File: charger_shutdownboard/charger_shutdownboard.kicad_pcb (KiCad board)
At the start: 2 copper layers, 53.5 x 58 mm, 18 parts, among them J1 Conn_01x08_Pin, J2 Conn_01x02_Pin, J3 Conn_01x02_Pin, J4 Conn_01x02_Pin, J5 Conn_01x02_Pin, J6 Conn_01x02_Pin, J7 Conn_01x02_Pin

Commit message: value for voltage divider resistors for bspd_fault changed
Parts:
- R1: value 70k -> 68k
- R2: value 50k -> 47k
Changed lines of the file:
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@@
 		)
 		(fp_text user "${REFERENCE}"
-			(at 3.54 6.25 360)
+			(at 3.54 6.25 0)
 			(layer "F.Fab")
 			(effects
@@
 		(tags "connector Molex Nano-Fit side entry")
 		(property "Reference" "J4"
-			(at 0 -2.92 360)
+			(at 0 -2.92 0)
 			(layer "F.SilkS")
 			(effects
@@
 		)
 		(property "Value" "Conn_01x02_Pin"
-			(at 0 5.42 360)
+			(at 0 5.42 0)
 			(layer "F.Fab")
 			(effects
@@
 			)
 		)
-		(property "Value" "70k"
+		(property "Value" "68k"
 			(at 0 1.65 0)
 			(layer "F.Fab")
@@
 		(tags "connector Molex Nano-Fit side entry")
 		(property "Reference" "J3"
-			(at 0 -2.92 360)
+			(at 0 -2.92 0)
 			(layer "F.SilkS")
 			(effects
@@
 		)
 		(property "Value" "Conn_01x02_Pin"
-			(at 0 5.42 360)
+			(at 0 5.42 0)
 			(layer "F.Fab")
 			(effects
@@
 		(tags "resistor handsolder")
 		(property "Reference" "R4"
-			(at 0 -2 360)
+			(at 0 -2 0)
 			(layer "F.SilkS")
 			(effects
@@
 		)
 		(property "Value" "38k"
-			(at 0 1.65 360)
+			(at 0 1.65 0)
 			(layer "F.Fab")
 			(effects
@@
 		)
 		(fp_text user "${REFERENCE}"
-			(at 0 0 360)
+			(at 0 0 0)
 			(layer "F.Fab")
 			(effects
@@
 		)
 		(fp_text user "${REFERENCE}"
-			(at 1.1 1.25 360)
+			(at 1.1 1.25 0)
 			(layer "F.Fab")
 			(effects
@@
 		(tags "resistor handsolder")
 		(property "Reference" "R2"
-			(at 0 -2 360)
+			(at 0 -2 0)
 			(layer "F.SilkS")
 			(effects
@@
 			)
 		)
-		(property "Value" "50k"
-			(at 0 1.65 360)
+		(property "Value" "47k"
+			(at 0 1.65 0)
 			(layer "F.Fab")
 			(effects
@@
 		)
 		(fp_text user "${REFERENCE}"
-			(at 0 0 360)
+			(at 0 0 0)
 			(layer "F.Fab")
 			(effects
@@
 		(tags "connector Molex Nano-Fit side entry")
 		(property "Reference" "J6"
-			(at 0 -2.92 360)
+			(at 0 -2.92 0)
 			(layer "F.SilkS")
 			(effects
@@
 		)
 		(property "Value" "Conn_01x02_Pin"
-			(at 0 5.42 360)
+			(at 0 5.42 0)
 			(layer "F.Fab")
 			(effects

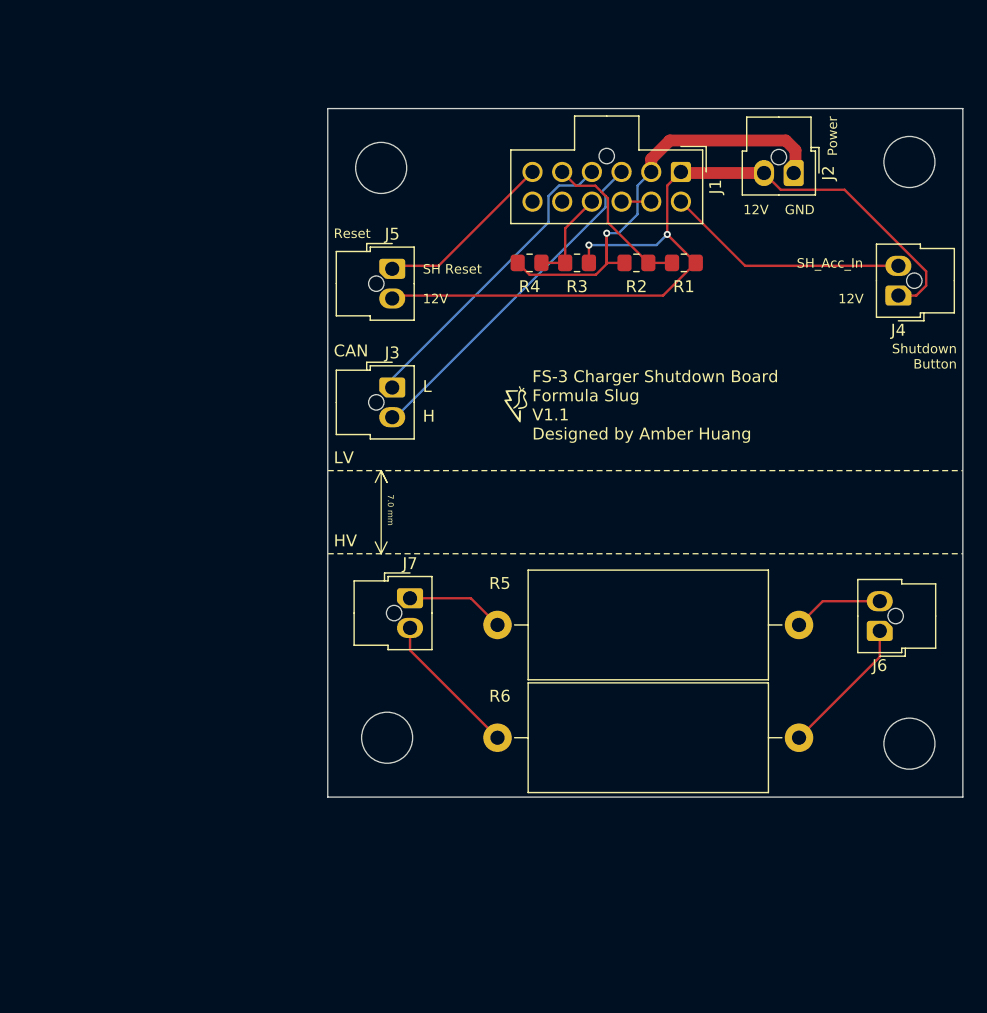
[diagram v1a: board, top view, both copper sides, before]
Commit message: Revised PCB for J1772 negotiation
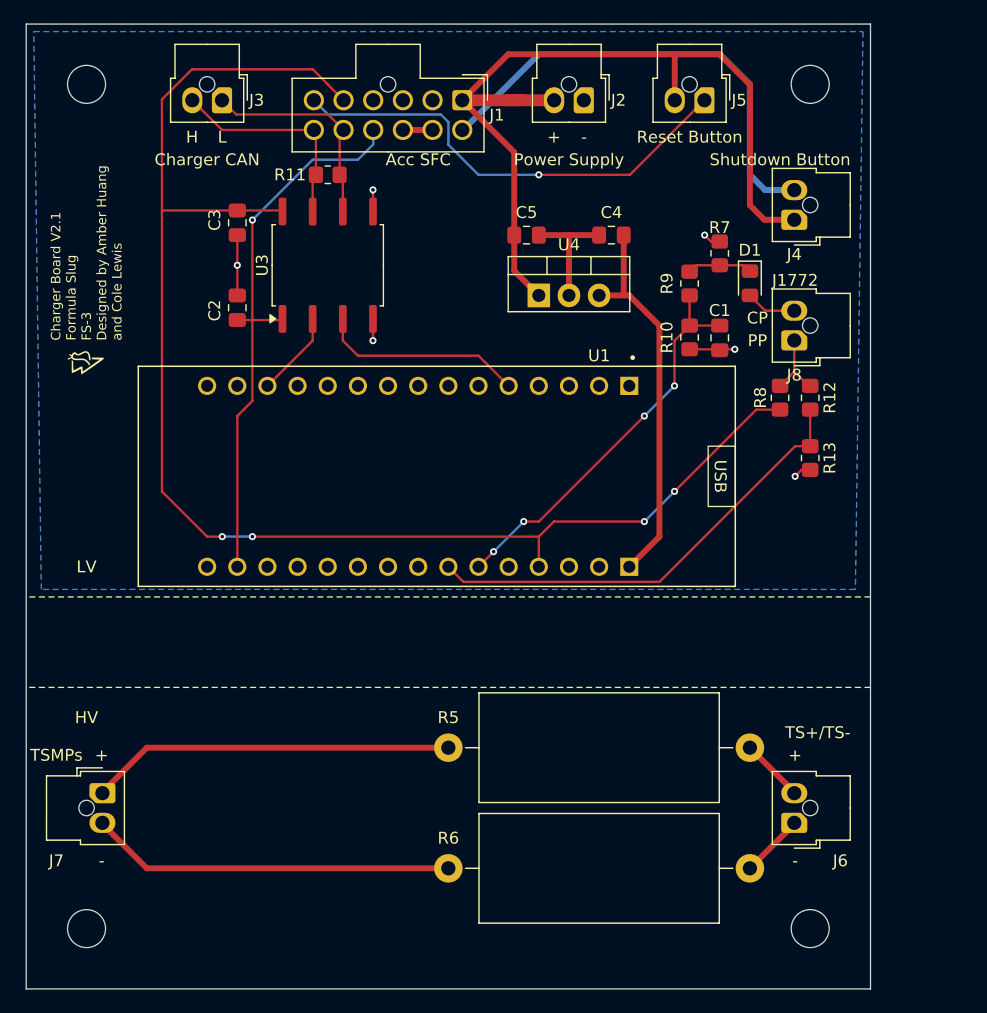
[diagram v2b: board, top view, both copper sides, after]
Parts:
- removed R1: 68k, Resistor_SMD:R_0805_2012Metric_Pad1.20x1.40mm_HandSolder
- removed R2: 47k, Resistor_SMD:R_0805_2012Metric_Pad1.20x1.40mm_HandSolder
- removed R3: 100k, Resistor_SMD:R_0805_2012Metric_Pad1.20x1.40mm_HandSolder
- removed R4: 38k, Resistor_SMD:R_0805_2012Metric_Pad1.20x1.40mm_HandSolder
- removed the REF** at (176.0, 116.5)
- removed the REF** at (132.0, 116.0)
- removed the REF** at (131.5, 68.0)
- removed the REF** at (176.0, 67.5)
- added C1: 100nF, Capacitor_SMD:C_0805_2012Metric_Pad1.18x1.45mm_HandSolder, F.Cu at (160.0, 82.3)
- added C2: 100nF, Capacitor_SMD:C_0805_2012Metric_Pad1.18x1.45mm_HandSolder, F.Cu at (119.4, 79.8)
- added C3: 100nF, Capacitor_SMD:C_0805_2012Metric_Pad1.18x1.45mm_HandSolder, F.Cu at (119.4, 72.6)
- added C4: 100nF, Capacitor_SMD:C_0805_2012Metric_Pad1.18x1.45mm_HandSolder, F.Cu at (150.9, 73.7)
- added C5: 100nF, Capacitor_SMD:C_0805_2012Metric_Pad1.18x1.45mm_HandSolder, F.Cu at (143.7, 73.7)
- added D1: D, Diode_SMD:D_0805_2012Metric_Pad1.15x1.40mm_HandSolder, F.Cu at (162.6, 77.7)
- added J8: J1772, Connector_Molex:Molex_Nano-Fit_105309-xx02_1x02_P2.50mm_Vertical, F.Cu at (166.3, 82.5)
- added R10: 499k, Resistor_SMD:R_0805_2012Metric_Pad1.20x1.40mm_HandSolder, F.Cu at (157.5, 82.3)
- added R11: 120, Resistor_SMD:R_0805_2012Metric_Pad1.20x1.40mm_HandSolder, F.Cu at (127.0, 68.6)
- added R12: 200k, Resistor_SMD:R_0805_2012Metric_Pad1.20x1.40mm_HandSolder, F.Cu at (167.6, 87.4)
- added R13: 330k, Resistor_SMD:R_0805_2012Metric_Pad1.20x1.40mm_HandSolder, F.Cu at (167.6, 92.4)
- added R7: 866, Resistor_SMD:R_0805_2012Metric_Pad1.20x1.40mm_HandSolder, F.Cu at (160.0, 75.2)
- added R8: 330, Resistor_SMD:R_0805_2012Metric_Pad1.20x1.40mm_HandSolder, F.Cu at (165.1, 87.4)
- added R9: 330k, Resistor_SMD:R_0805_2012Metric_Pad1.20x1.40mm_HandSolder, F.Cu at (157.5, 77.7)
- added REF**: MountingHole_3.2mm_M3, MountingHole:MountingHole_3.2mm_M3, F.Cu at (106.7, 132.1)
- added REF**: MountingHole_3.2mm_M3, MountingHole:MountingHole_3.2mm_M3, F.Cu at (167.6, 61.0)
- added REF**: MountingHole_3.2mm_M3, MountingHole:MountingHole_3.2mm_M3, F.Cu at (167.6, 132.1)
- added REF**: MountingHole_3.2mm_M3, MountingHole:MountingHole_3.2mm_M3, F.Cu at (106.7, 61.0)
- added U1: NUCLEO-L432KC, FS_3_Global_Footprint_Library:NUCLEO-L432KC, F.Cu at (136.2, 94.0)
- added U3: ISO1050DUB, Package_SO:SOP-8_6.62x9.15mm_P2.54mm, F.Cu at (127.0, 76.2)
- added U4: LM7809_TO220, Package_TO_SOT_THT:TO-220-3_Vertical, F.Cu at (144.8, 78.7)
- J1: value Conn_01x08_Pin -> Acc SFC
- J2: value Conn_01x02_Pin -> Power Supply
- J3: value Conn_01x02_Pin -> Charger CAN
- J4: value Conn_01x02_Pin -> Shutdown Button
- J5: value Conn_01x02_Pin -> Reset Button
- J6: value Conn_01x02_Pin -> TS+/TS-
- J7: value Conn_01x02_Pin -> TSMPs
- moved G*** 39.9 mm to (106.7, 81.2), turned to 90 degrees
- moved J7 30.7 mm to (108.0, 120.7)
- moved J5 29.9 mm to (158.7, 62.3), turned to -90 degrees
- moved J3 28.1 mm to (118.1, 62.3), turned to -90 degrees
- moved J1 19.4 mm to (138.3, 62.3)
- moved J2 18.7 mm to (148.6, 62.3)
- moved J6 17.7 mm to (166.3, 123.2)
- moved R6 11.8 mm to (137.2, 127.0)
- moved R5 11.1 mm to (137.2, 116.8)
- moved J4 10.8 mm to (166.3, 72.4)
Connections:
- J1 pad 10: /Charge_State -> +3V3
- J1 pad 11: unconnected-(J1-Pin_11-Pad11) -> /CAN_L
- J1 pad 12: unconnected-(J1-Pin_12-Pad12) -> /CAN_H
- J1 pad 3: /CAN_H -> unconnected-(J1-Pin_3-Pad3)
- J1 pad 4: /CAN_L -> unconnected-(J1-Pin_4-Pad4)
- J1 pad 5: /BSPD_fault -> +5V
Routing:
- net +5V: track 0.00 -> 121.1 mm, vias 0 -> 4
- net +3V3: track 0.00 -> 47.5 mm, vias 0 -> 1
- net /Proximity_Pilot_Filtered: track 0.00 -> 38.8 mm
- net /Control_Pilot_Filtered: track 0.00 -> 33.5 mm, vias 0 -> 4
- net +9V: track 0.00 -> 32.6 mm
- net /Shutdown_Reset: track 15.1 -> 39.2 mm, vias 0 -> 1
- net Net-(J7-Pin_1): track 8.30 -> 30.7 mm
- net /Shutdown_Acc_In: track 20.6 -> 39.7 mm
- net Net-(J7-Pin_2): track 12.3 -> 30.7 mm
- net /CAN_TX: track 0.00 -> 17.4 mm
- net /BSPD_fault: track 13.6 -> 0.00 mm
- net GND: track 38.4 -> 25.7 mm, vias 1 -> 6
- net /CAN_H: track 29.1 -> 17.7 mm
- net /Charge_State: track 8.09 -> 0.00 mm
- net /CAN_L: track 25.3 -> 17.6 mm
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- added copper zone on B.Cu, net GND
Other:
- board size 53.5 x 58 mm -> 71.1 x 81.3 mm
- board text added: "${TITLE} V${REVISION} ${COMPANY} FS-3 Designed by Amber Huang and Cole Lewis"
- board text added: "+"
- board text added: "-"
- board text added: "CP"
- board text added: "PP"
- board text removed: "12V"
- board text removed: "7.0 mm"
- board text removed: "CAN"
- board text removed: "FS-3 Charger Shutdown Board Formula Slug V1.1 Designed by Amber Huang"
- board text removed: "GND"
- board text removed: "Power"
- board text removed: "Reset"
- board text removed: "SH Reset"
- board text removed: "SH_Acc_In"
- board text removed: "Shutdown Button"
